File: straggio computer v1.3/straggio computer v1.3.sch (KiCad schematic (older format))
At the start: 0 parts

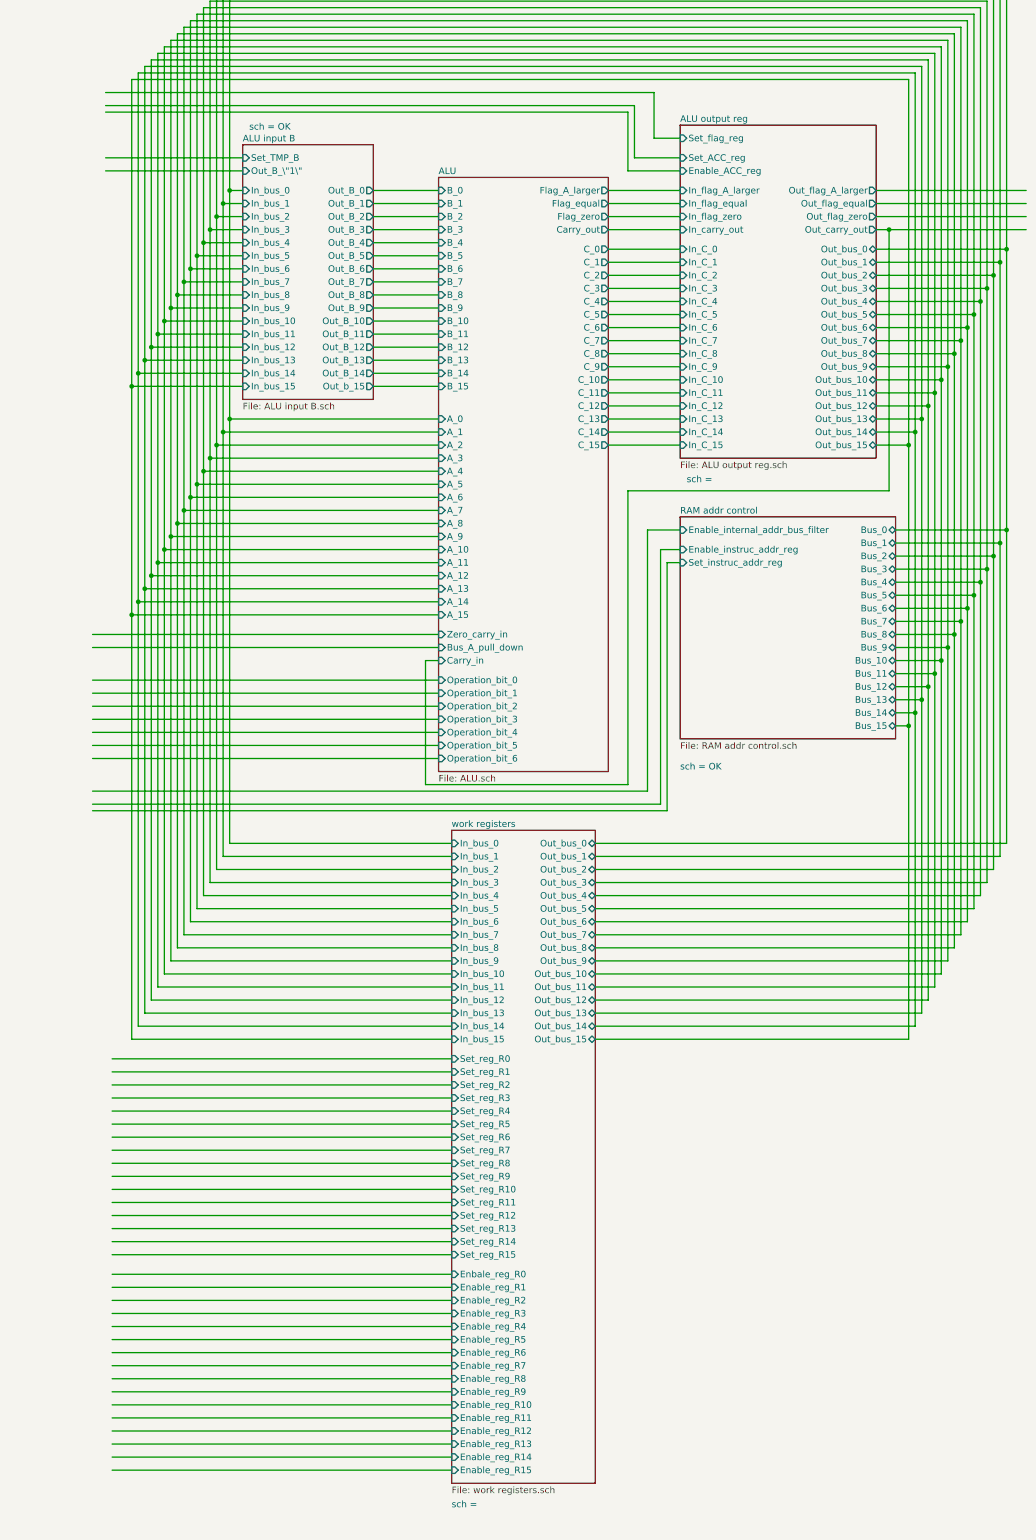
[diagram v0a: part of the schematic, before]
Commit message: update
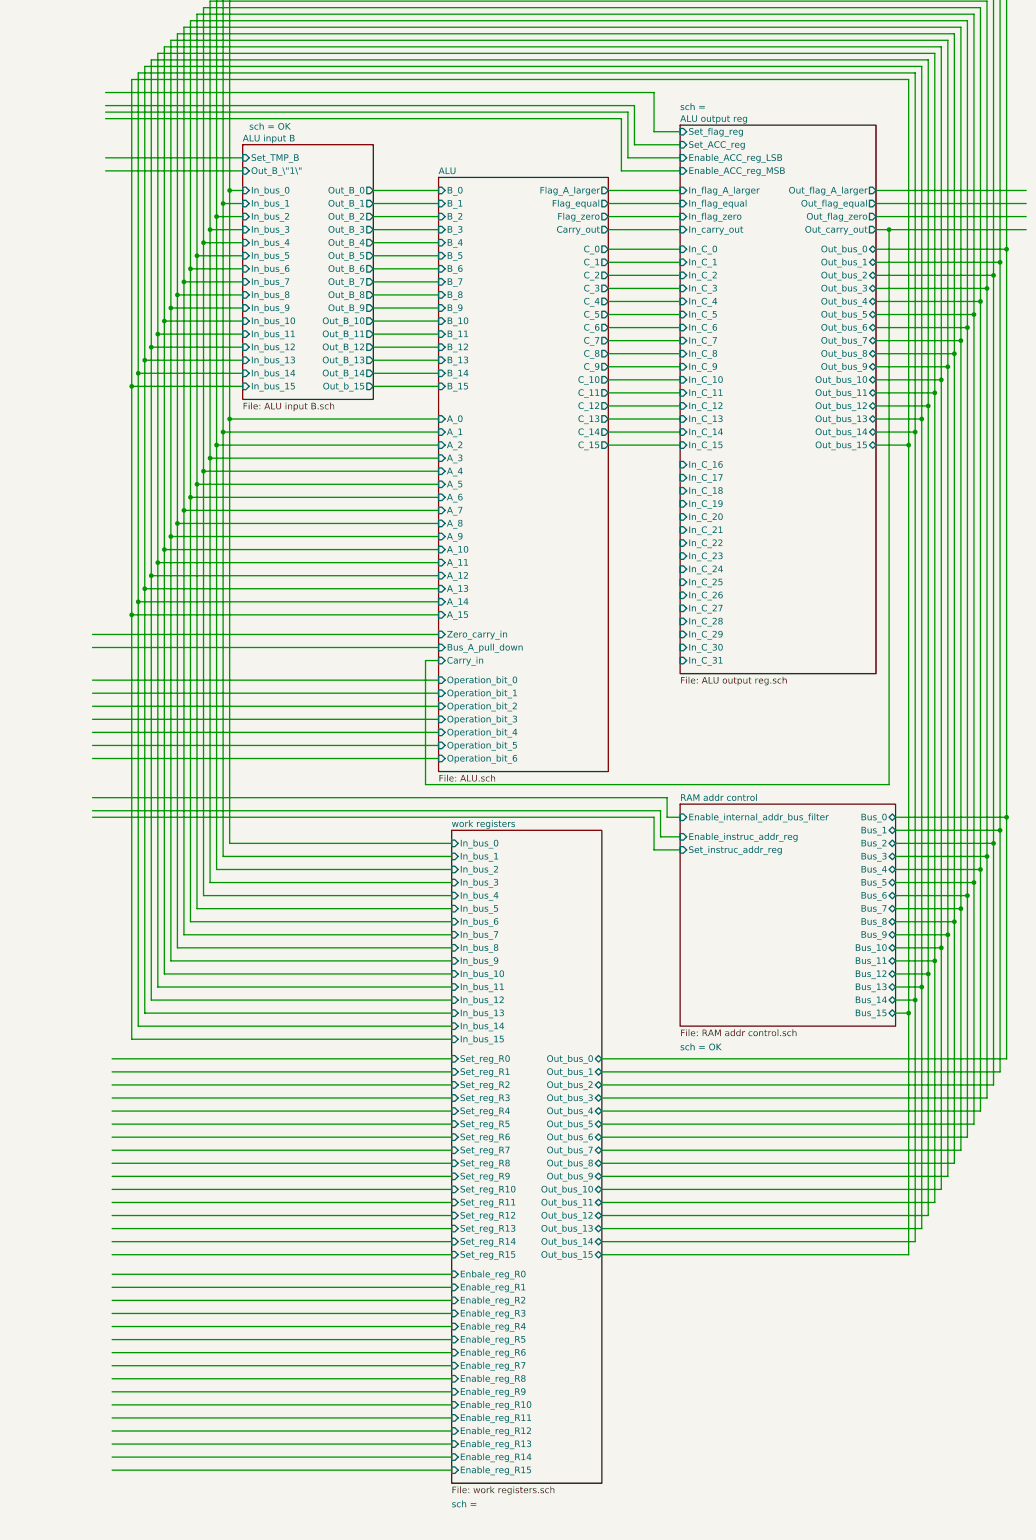
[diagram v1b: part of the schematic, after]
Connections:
- wire segments 316 -> 317
